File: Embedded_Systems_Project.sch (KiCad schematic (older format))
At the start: 1 part

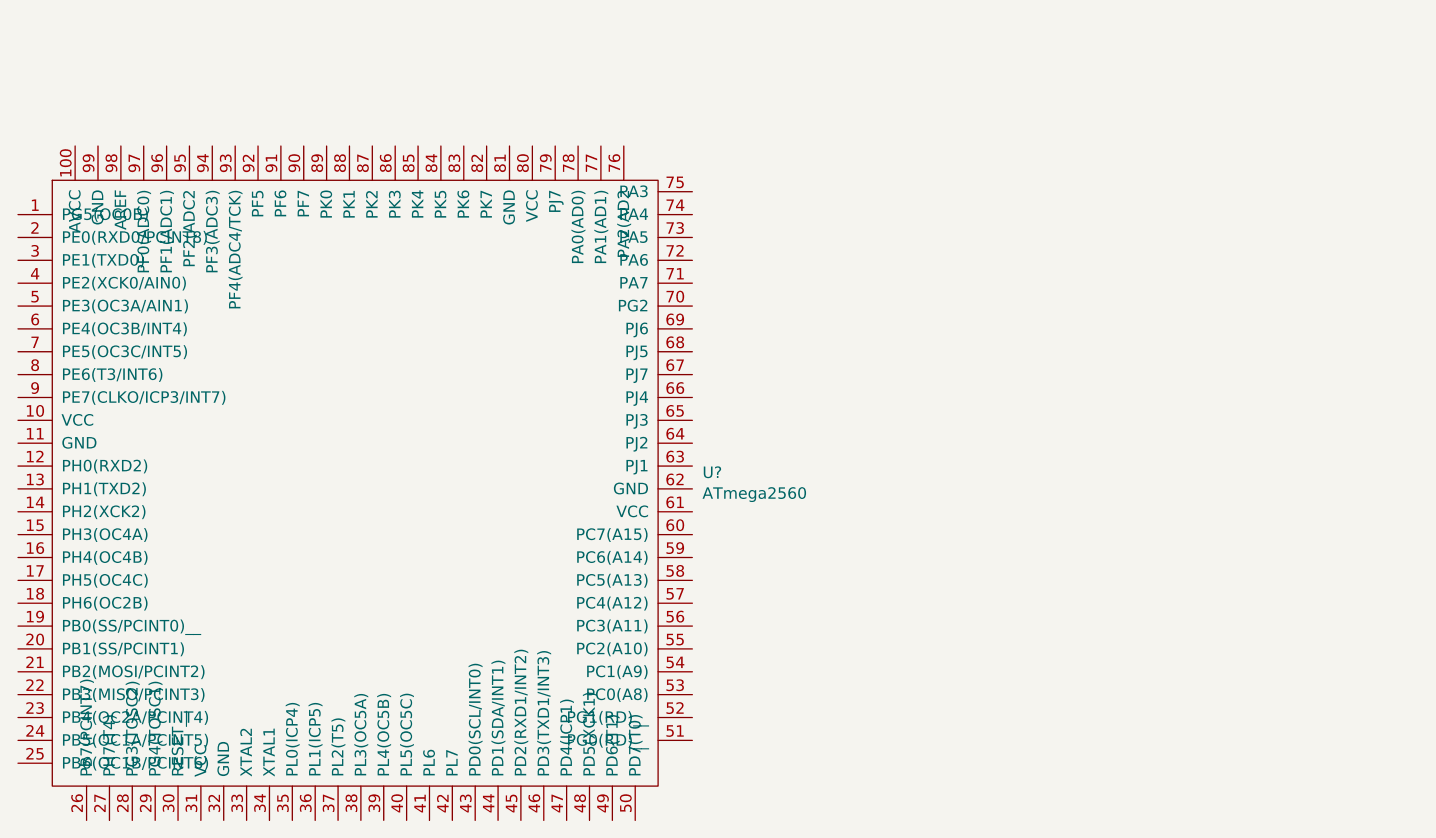
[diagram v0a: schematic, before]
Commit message: added footprint
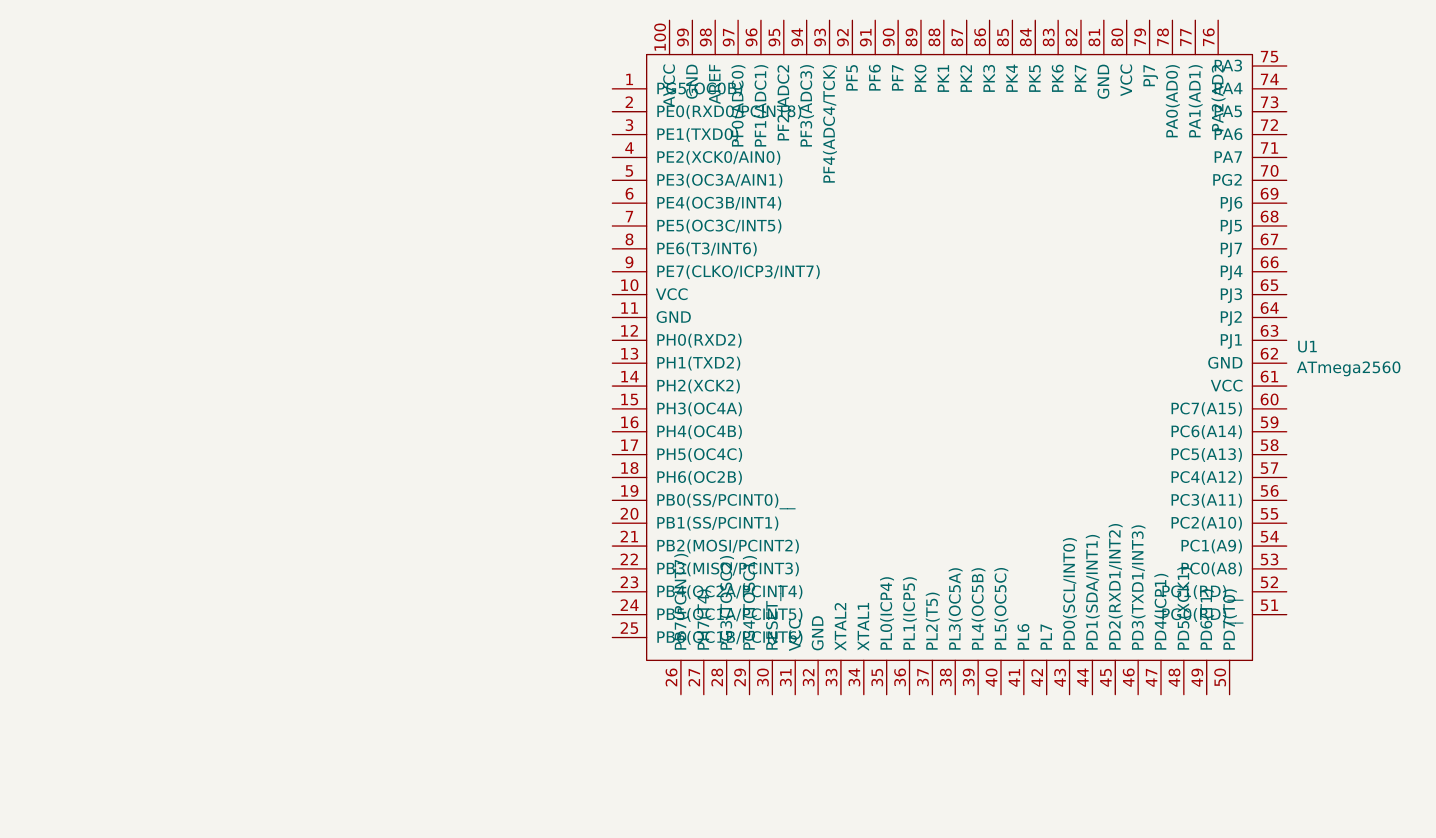
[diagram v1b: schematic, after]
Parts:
- U1: renamed from U?; footprint (none) -> Package_QFP:TQFP-100_14x14mm_P0.5mm
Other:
- moved on the sheet: U1
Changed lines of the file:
@@
 $EndDescr
 $Comp
-L ATmega2560:ATmega2560 U?
+L ATmega2560:ATmega2560 U1
 U 1 1 606C76A0
-P 5200 3750
-F 0 "U?" H 6744 3921 50  0000 L CNN
-F 1 "ATmega2560" H 6744 3830 50  0000 L CNN
-F 2 "" H 3100 6850 50  0001 C CNN
-F 3 "" H 3100 6850 50  0001 C CNN
-	1    5200 3750
+P 7800 3200
+F 0 "U1" H 9344 3371 50  0000 L CNN
+F 1 "ATmega2560" H 9344 3280 50  0000 L CNN
+F 2 "Package_QFP:TQFP-100_14x14mm_P0.5mm" H 5700 6300 50  0001 C CNN
+F 3 "https://ww1.microchip.com/downloads/en/DeviceDoc/ATmega640-1280-1281-2560-2561-Datasheet-DS40002211A.pdf" H 5700 6300 50  0001 C CNN
+	1    7800 3200
 	1    0    0    -1
 $EndComp
